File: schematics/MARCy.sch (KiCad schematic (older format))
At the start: 3 parts, among them J2 JTAG, U3 XC9572XL-TQ100

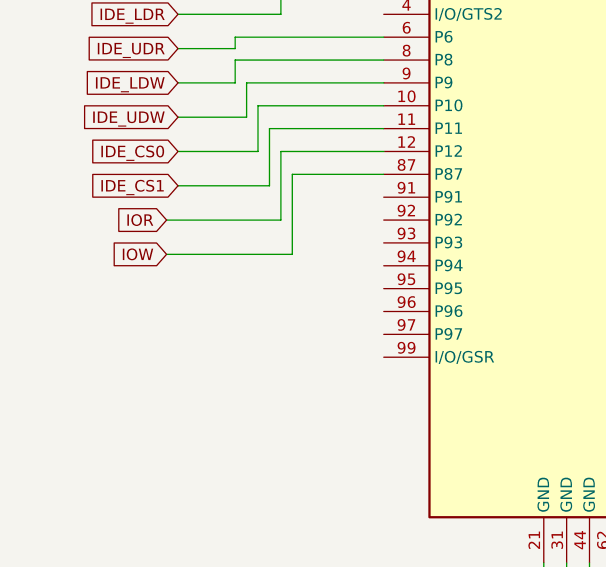
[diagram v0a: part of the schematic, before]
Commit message: Added missing FDC control signals.
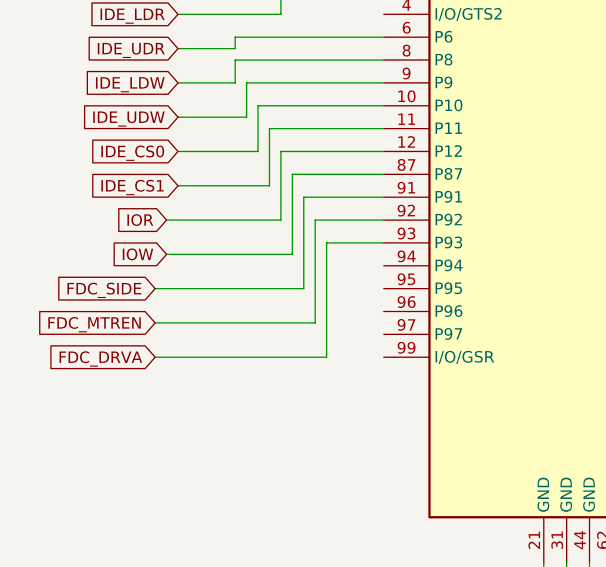
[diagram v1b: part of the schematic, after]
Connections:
- net FDC_SIDE: now reaches U3.91 (P91)
- net FDC_MTREN: now reaches U3.92 (P92)
- net FDC_DRVA: now reaches U3.93 (P93)
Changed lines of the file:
@@
 Wire Wire Line
 	2950 5200 2400 5200
+Text GLabel 2350 5350 0    50   Input ~ 0
+FDC_SIDE
+Text GLabel 2350 5500 0    50   Input ~ 0
+FDC_MTREN
+Text GLabel 2350 5650 0    50   Input ~ 0
+FDC_DRVA
+Wire Wire Line
+	3350 4950 3000 4950
+Wire Wire Line
+	3000 4950 3000 5350
+Wire Wire Line
+	3000 5350 2350 5350
+Wire Wire Line
+	3050 5050 3050 5500
+Wire Wire Line
+	3050 5500 2350 5500
+Wire Wire Line
+	3050 5050 3350 5050
+Wire Wire Line
+	3350 5150 3100 5150
+Wire Wire Line
+	3100 5150 3100 5650
+Wire Wire Line
+	3100 5650 2350 5650
 Wire Bus Line
 	5600 1950 5600 3450

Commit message: Fixes to FDC signal mapping.
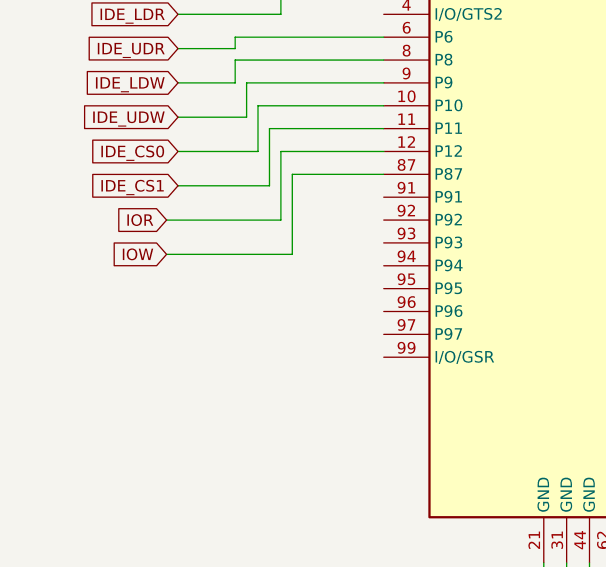
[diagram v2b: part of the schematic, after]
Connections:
- net FDC_DRVA: no longer names the net of U3.93 (P93)
- net FDC_MTREN: no longer names the net of U3.92 (P92)
- net FDC_SIDE: no longer names the net of U3.91 (P91)
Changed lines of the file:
@@
 Wire Wire Line
 	2950 5200 2400 5200
-Text GLabel 2350 5350 0    50   Input ~ 0
-FDC_SIDE
-Text GLabel 2350 5500 0    50   Input ~ 0
-FDC_MTREN
-Text GLabel 2350 5650 0    50   Input ~ 0
-FDC_DRVA
-Wire Wire Line
-	3350 4950 3000 4950
-Wire Wire Line
-	3000 4950 3000 5350
-Wire Wire Line
-	3000 5350 2350 5350
-Wire Wire Line
-	3050 5050 3050 5500
-Wire Wire Line
-	3050 5500 2350 5500
-Wire Wire Line
-	3050 5050 3350 5050
-Wire Wire Line
-	3350 5150 3100 5150
-Wire Wire Line
-	3100 5150 3100 5650
-Wire Wire Line
-	3100 5650 2350 5650
 Wire Bus Line
 	5600 1950 5600 3450
